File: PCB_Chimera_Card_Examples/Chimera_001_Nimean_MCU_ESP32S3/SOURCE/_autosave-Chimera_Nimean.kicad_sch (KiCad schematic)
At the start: 14 parts, among them CN1 NASB0-S6701-TS50, SW1 K2-1107ST-A4SW-06, SW2 K2-1107ST-A4SW-06, U1 ESP32-S3-WROOM-1-N8

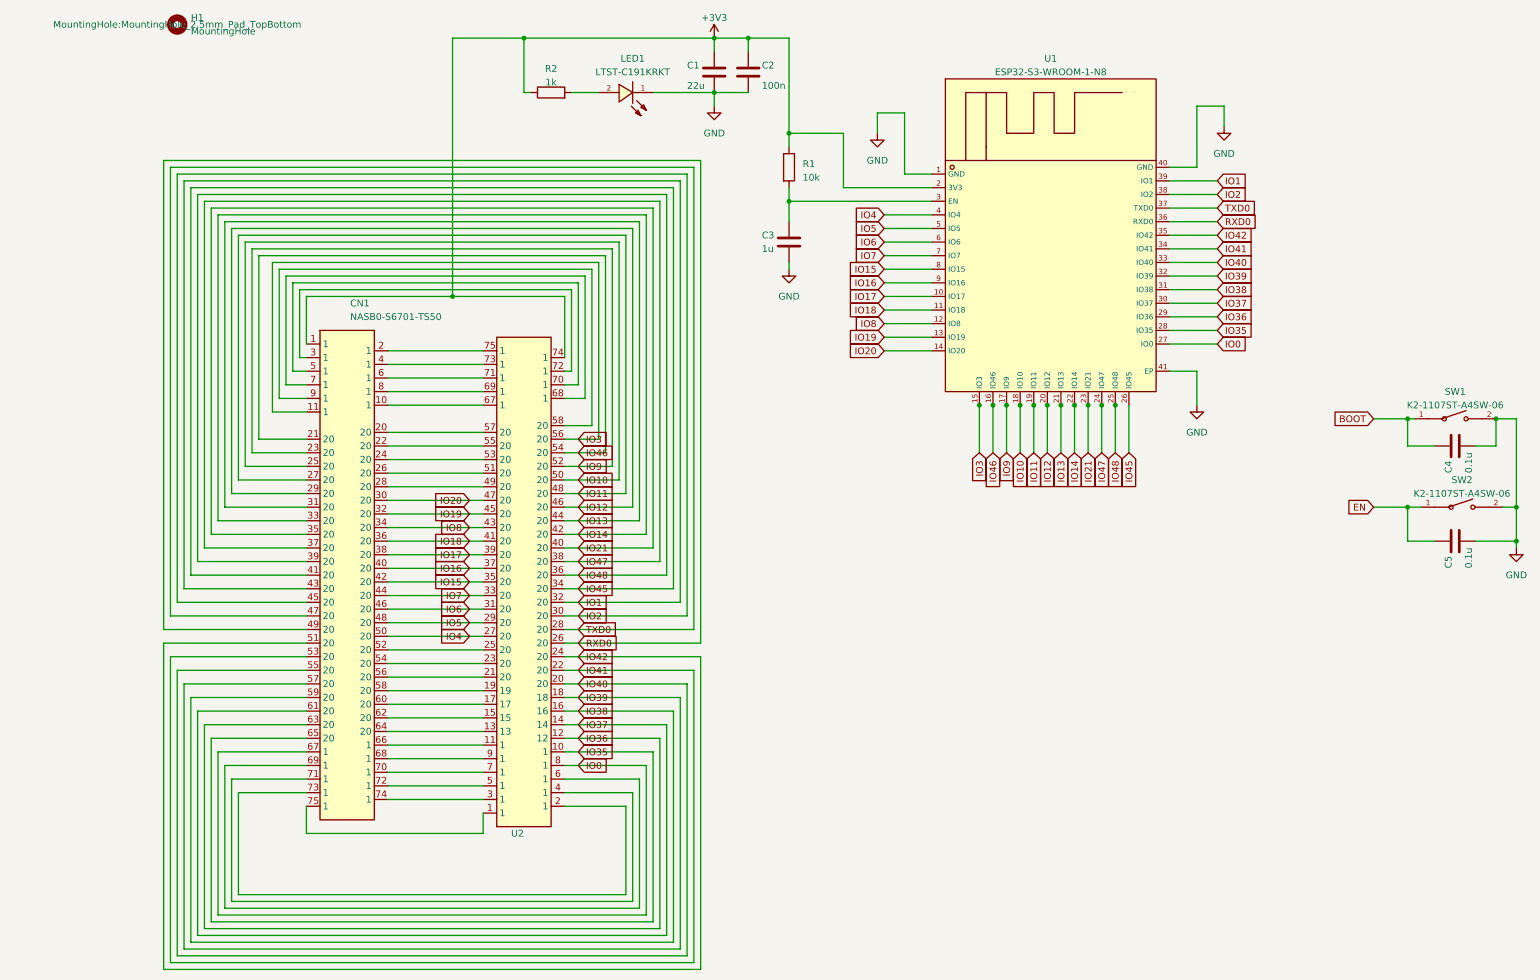
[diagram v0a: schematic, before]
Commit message: Added Nimean Pin description document
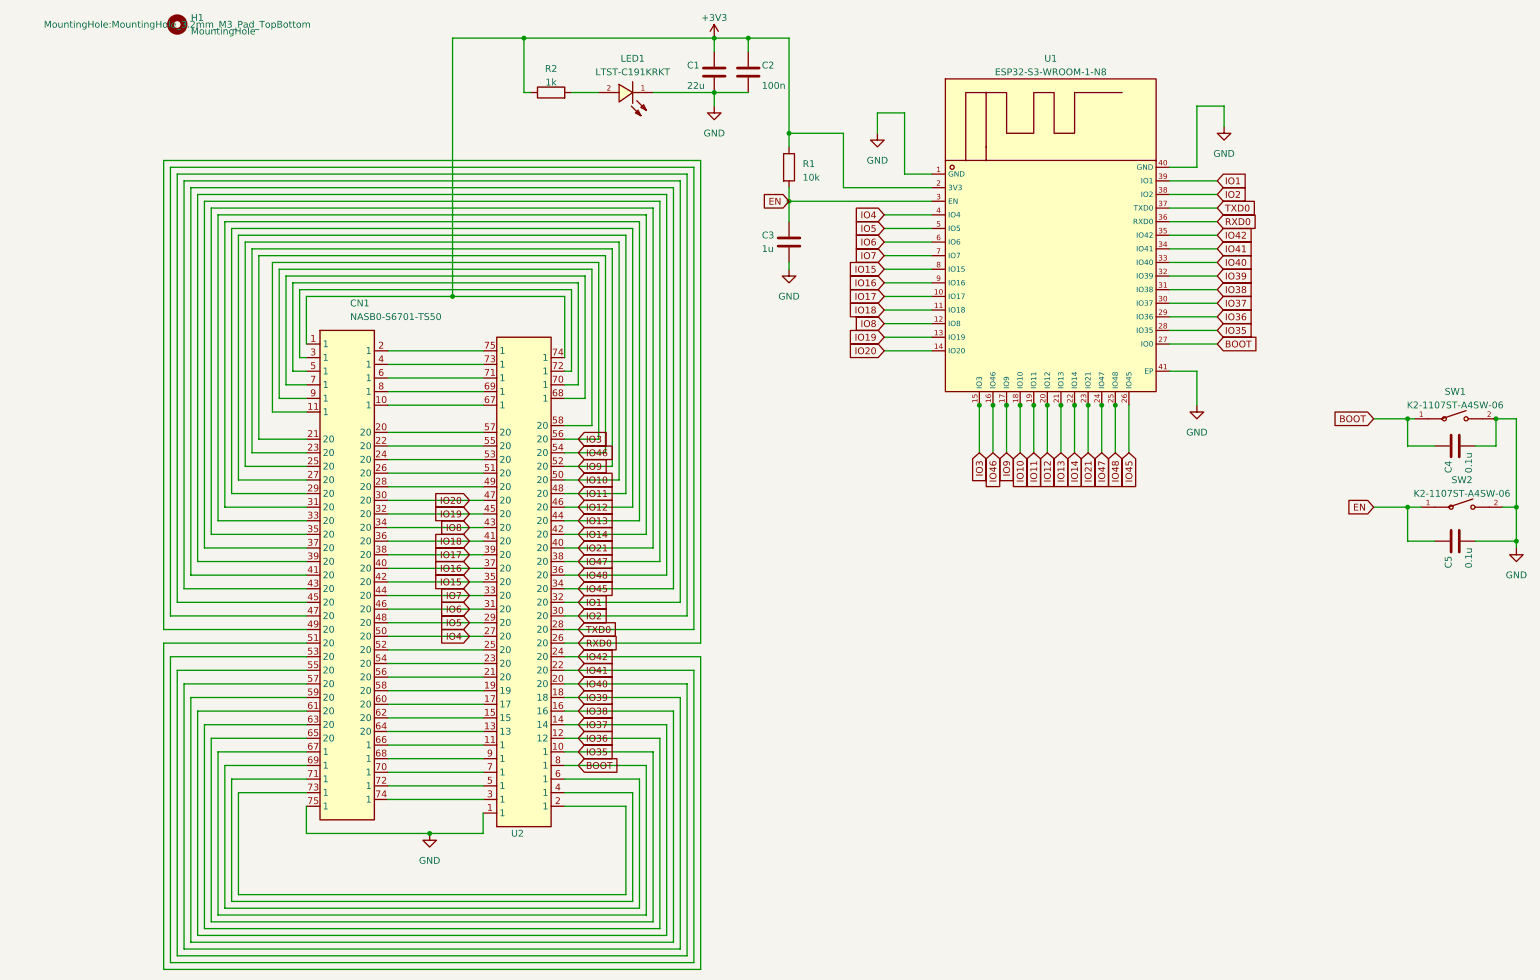
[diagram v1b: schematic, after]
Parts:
- H1: footprint MountingHole:MountingHole_2.5mm_Pad_TopBottom -> MountingHole:MountingHole_3.2mm_M3_Pad_TopBottom
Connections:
- net IO0 is gone; now on net BOOT: CN1.67 (1), U1.27 (IO0), U2.8 (1)
- net EN: now also C3.1, R1.2, U1.3 (EN)
- net GND: now also CN1.75 (1), U2.1
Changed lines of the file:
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@@
   (junction (at 132.08 38.1) (diameter 0) (color 0 0 0 0)
   )
+  (junction (at 64.9376 168.91) (diameter 0) (color 0 0 0 0)
+  )
   (junction (at 82.55 20.32) (diameter 0) (color 0 0 0 0)
   )
@@
     (stroke (width 0) (type default))
   )
+  (wire (pts (xy 64.9376 168.91) (xy 74.93 168.91))
+    (stroke (width 0) (type default))
+  )
   (wire (pts (xy 115.57 194.31) (xy 115.57 135.89))
     (stroke (width 0) (type default))
@@
     (stroke (width 0) (type default))
   )
-  (wire (pts (xy 41.91 168.91) (xy 74.93 168.91))
+  (wire (pts (xy 41.91 168.91) (xy 64.9376 168.91))
     (stroke (width 0) (type default))
   )
@@
     )
   )
-  (global_label "IO0" (shape input) (at 92.71 156.21 0) (fields_autoplaced)
-    (effects (font (size 1.27 1.27)) (justify left))
-    (property "Intersheetrefs" "${INTERSHEET_REFS}" (at 98.7606 156.21 0)
+  (global_label "BOOT" (shape input) (at 92.71 156.21 0) (fields_autoplaced)
+    (effects (font (size 1.27 1.27)) (justify left))
+    (property "Intersheetrefs" "${INTERSHEET_REFS}" (at 100.5144 156.21 0)
       (effects (font (size 1.27 1.27)) (justify left) hide)
     )
@@
     )
   )
+  (global_label "EN" (shape input) (at 132.08 50.8 180) (fields_autoplaced)
+    (effects (font (size 1.27 1.27)) (justify right))
+    (property "Intersheetrefs" "${INTERSHEET_REFS}" (at 126.6947 50.8 0)
+      (effects (font (size 1.27 1.27)) (justify right) hide)
+    )
+  )
   (global_label "IO35" (shape input) (at 92.71 153.67 0) (fields_autoplaced)
     (effects (font (size 1.27 1.27)) (justify left))
@@
     )
   )
-  (global_label "IO0" (shape input) (at 212.09 77.47 0) (fields_autoplaced)
-    (effects (font (size 1.27 1.27)) (justify left))
-    (property "Intersheetrefs" "${INTERSHEET_REFS}" (at 218.1406 77.47 0)
+  (global_label "BOOT" (shape input) (at 212.09 77.47 0) (fields_autoplaced)
+    (effects (font (size 1.27 1.27)) (justify left))
+    (property "Intersheetrefs" "${INTERSHEET_REFS}" (at 219.8944 77.47 0)
       (effects (font (size 1.27 1.27)) (justify left) hide)
     )
@@
     (pin "2")
     (instances
-      (project "Card_ESP32"
+      (project "Chimera_Nimean"
         (path "/9df5003c-5fc3-47df-88fb-9e33c833ceef"
           (reference "SW2") (unit 1)
@@
     (pin "9")
     (instances
-      (project "Card_ESP32"
+      (project "Chimera_Nimean"
         (path "/9df5003c-5fc3-47df-88fb-9e33c833ceef"
           (reference "U2") (unit 1)
@@
     (pin "2")
     (instances
-      (project "Card_ESP32"
+      (project "Chimera_Nimean"
         (path "/9df5003c-5fc3-47df-88fb-9e33c833ceef"
           (reference "C3") (unit 1)
@@
     (pin "9")
     (instances
-      (project "Card_ESP32"
+      (project "Chimera_Nimean"
         (path "/9df5003c-5fc3-47df-88fb-9e33c833ceef"
           (reference "U1") (unit 1)
@@
     (pin "2")
     (instances
-      (project "Card_ESP32"
+      (project "Chimera_Nimean"
         (path "/9df5003c-5fc3-47df-88fb-9e33c833ceef"
           (reference "C4") (unit 1)
@@
     (pin "1")
     (instances
-      (project "Card_ESP32"
+      (project "Chimera_Nimean"
         (path "/9df5003c-5fc3-47df-88fb-9e33c833ceef"
           (reference "#PWR07") (unit 1)
@@
     (pin "2")
     (instances
-      (project "Card_ESP32"
+      (project "Chimera_Nimean"
         (path "/9df5003c-5fc3-47df-88fb-9e33c833ceef"
           (reference "C5") (unit 1)
@@
     (pin "2")
     (instances
-      (project "Card_ESP32"
+      (project "Chimera_Nimean"
         (path "/9df5003c-5fc3-47df-88fb-9e33c833ceef"
           (reference "C1") (unit 1)
@@
     (pin "1")
     (instances
-      (project "Card_ESP32"
+      (project "Chimera_Nimean"
         (path "/9df5003c-5fc3-47df-88fb-9e33c833ceef"
           (reference "#PWR06") (unit 1)
+        )
+      )
+    )
+  )
+  (symbol (lib_id "power:GND") (at 64.9376 168.91 0) (unit 1)
+    (in_bom yes) (on_board yes) (dnp no) (fields_autoplaced)
+    (property "Reference" "#PWR08" (at 64.9376 175.26 0)
+      (effects (font (size 1.27 1.27)) hide)
+    )
+    (property "Value" "GND" (at 64.9376 173.99 0)
+      (effects (font (size 1.27 1.27)))
+    )
+    (property "Footprint" "" (at 64.9376 168.91 0)
+      (effects (font (size 1.27 1.27)) hide)
+    )
+    (property "Datasheet" "" (at 64.9376 168.91 0)
+      (effects (font (size 1.27 1.27)) hide)
+    )
+    (pin "1")
+    (instances
+      (project "Chimera_Nimean"
+        (path "/9df5003c-5fc3-47df-88fb-9e33c833ceef"
+          (reference "#PWR08") (unit 1)
         )
       )
@@
       (effects (font (size 1.27 1.27)) (justify left))
     )
-    (property "Footprint" "MountingHole:MountingHole_2.5mm_Pad_TopBottom" (at 17.78 17.78 0)
+    (property "Footprint" "MountingHole:MountingHole_3.2mm_M3_Pad_TopBottom" (at 17.78 17.78 0)
       (effects (font (size 1.27 1.27)))
     )
@@
     )
     (instances
-      (project "Card_ESP32"
+      (project "Chimera_Nimean"
         (path "/9df5003c-5fc3-47df-88fb-9e33c833ceef"
           (reference "H1") (unit 1)
@@
     (pin "2")
     (instances
-      (project "Card_ESP32"
+      (project "Chimera_Nimean"
         (path "/9df5003c-5fc3-47df-88fb-9e33c833ceef"
           (reference "R2") (unit 1)
@@
     (pin "9")
     (instances
-      (project "Card_ESP32"
+      (project "Chimera_Nimean"
         (path "/9df5003c-5fc3-47df-88fb-9e33c833ceef"
           (reference "CN1") (unit 1)
@@
     (pin "1")
     (instances
-      (project "Card_ESP32"
+      (project "Chimera_Nimean"
         (path "/9df5003c-5fc3-47df-88fb-9e33c833ceef"
           (reference "#PWR03") (unit 1)
@@
     (pin "1")
     (instances
-      (project "Card_ESP32"
+      (project "Chimera_Nimean"
         (path "/9df5003c-5fc3-47df-88fb-9e33c833ceef"
           (reference "#PWR05") (unit 1)
@@
     (pin "1")
     (instances
-      (project "Card_ESP32"
+      (project "Chimera_Nimean"
         (path "/9df5003c-5fc3-47df-88fb-9e33c833ceef"
           (reference "#PWR01") (unit 1)
@@
     (pin "2")
     (instances
-      (project "Card_ESP32"
+      (project "Chimera_Nimean"
         (path "/9df5003c-5fc3-47df-88fb-9e33c833ceef"
           (reference "LED1") (unit 1)
@@
     (pin "2")
     (instances
-      (project "Card_ESP32"
+      (project "Chimera_Nimean"
         (path "/9df5003c-5fc3-47df-88fb-9e33c833ceef"
           (reference "C2") (unit 1)
@@
     (pin "2")
     (instances
-      (project "Card_ESP32"
+      (project "Chimera_Nimean"
         (path "/9df5003c-5fc3-47df-88fb-9e33c833ceef"
           (reference "SW1") (unit 1)
@@
     (pin "2")
     (instances
-      (project "Card_ESP32"
+      (project "Chimera_Nimean"
         (path "/9df5003c-5fc3-47df-88fb-9e33c833ceef"
           (reference "R1") (unit 1)
@@
     (pin "1")
     (instances
-      (project "Card_ESP32"
+      (project "Chimera_Nimean"
         (path "/9df5003c-5fc3-47df-88fb-9e33c833ceef"
           (reference "#PWR04") (unit 1)
@@
     (pin "1")
     (instances
-      (project "Card_ESP32"
+      (project "Chimera_Nimean"
         (path "/9df5003c-5fc3-47df-88fb-9e33c833ceef"
           (reference "#PWR02") (unit 1)
